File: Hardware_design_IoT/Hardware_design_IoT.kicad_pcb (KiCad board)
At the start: 2 copper layers, 91.2 x 78.8 mm, 90 parts, among them J1 Barrel_Jack_Switch, J2 Prog/Debug, Q1 Q_NPN_BEC_BRT, Q2 Q_NPN_BEC_BRT, Q3 Q_NPN_BEC_BRT, SW1 Input_SW1, SW2 Input_SW2, SW3 PWRKEY_SW, U1 MP1584EN, U2 TLV70033_SOT23-5, U3 STM32L073RZTx, U4 LD39200DPUR, U5 SIM7600E-H, U6 TXB0104RGY, Y1 32.768kHz, Y2 8MHz

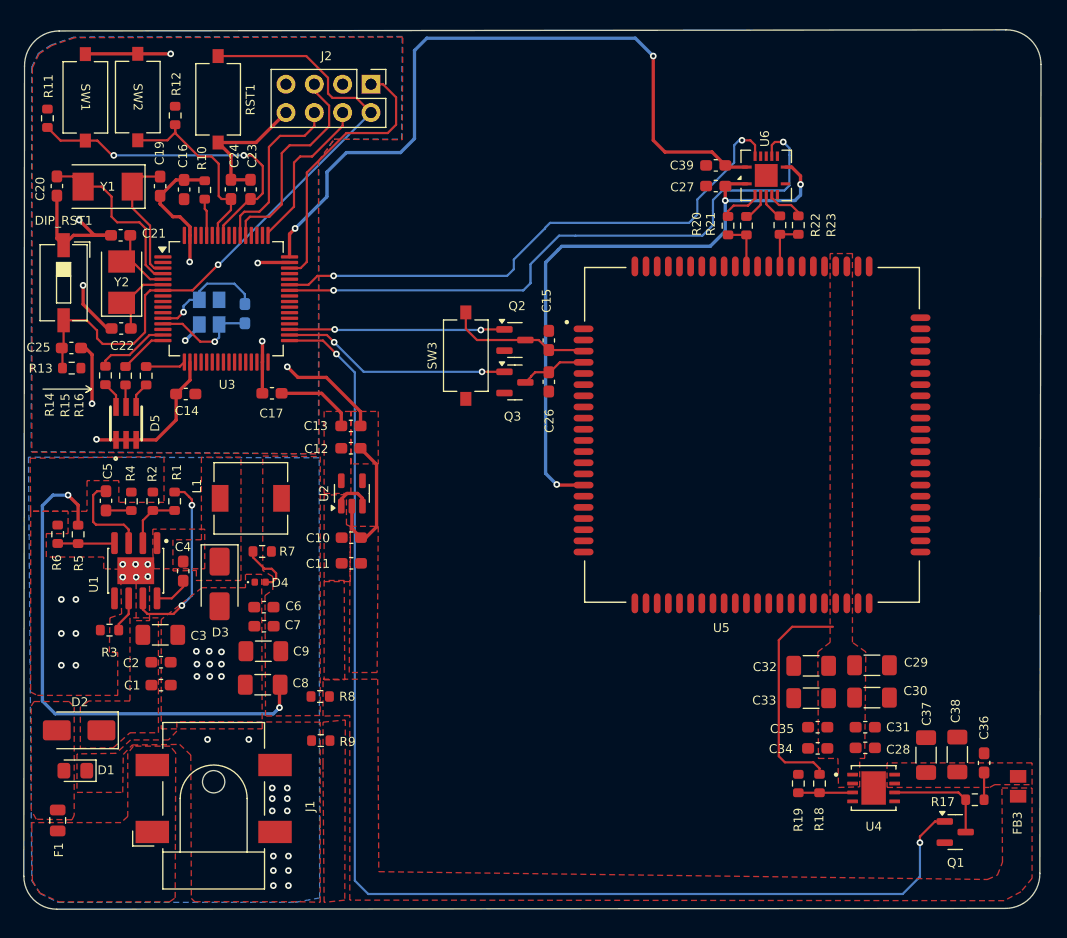
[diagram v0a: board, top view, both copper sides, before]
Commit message: Fin du projet
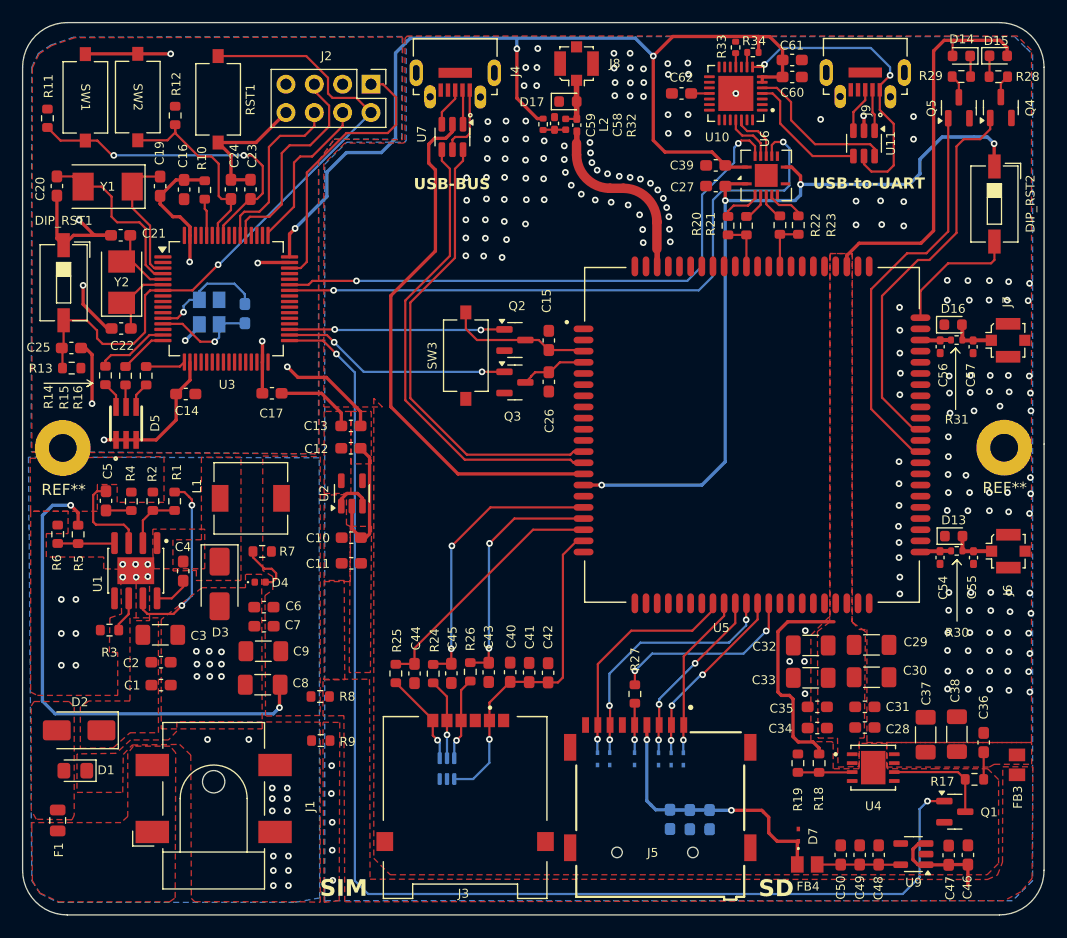
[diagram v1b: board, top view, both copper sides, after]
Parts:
- added C40: 100nF, Capacitor_SMD:C_0603_1608Metric_Pad1.08x0.95mm_HandSolder, F.Cu at (135.4, 116.5)
- added C41: 10nF, Capacitor_SMD:C_0603_1608Metric_Pad1.08x0.95mm_HandSolder, F.Cu at (137.1, 116.5)
- added C42: 10pF, Capacitor_SMD:C_0603_1608Metric_Pad1.08x0.95mm_HandSolder, F.Cu at (138.8, 116.5)
- added C43: 22pF, Capacitor_SMD:C_0603_1608Metric_Pad1.08x0.95mm_HandSolder, F.Cu at (133.5, 116.5)
- added C44: 22pF, Capacitor_SMD:C_0603_1608Metric_Pad1.08x0.95mm_HandSolder, F.Cu at (126.8, 116.6)
- added C45: 22pF, Capacitor_SMD:C_0603_1608Metric_Pad1.08x0.95mm_HandSolder, F.Cu at (130.2, 116.6)
- added C46: 0.1uF, Capacitor_SMD:C_0603_1608Metric_Pad1.08x0.95mm_HandSolder, F.Cu at (176.4, 132.8)
- added C47: 10uF, Capacitor_SMD:C_0603_1608Metric_Pad1.08x0.95mm_HandSolder, F.Cu at (174.7, 132.9)
- added C48: 10uF, Capacitor_SMD:C_0603_1608Metric_Pad1.08x0.95mm_HandSolder, F.Cu at (168.4, 132.8)
- added C49: 0.1uF, Capacitor_SMD:C_0603_1608Metric_Pad1.08x0.95mm_HandSolder, F.Cu at (166.8, 132.8)
- added C50: 22pF, Capacitor_SMD:C_0603_1608Metric_Pad1.08x0.95mm_HandSolder, F.Cu at (165.1, 132.8)
- added C51: 100nF, Capacitor_SMD:C_0603_1608Metric_Pad1.08x0.95mm_HandSolder, B.Cu at (151.5, 129.7)
- added C52: 10uF, Capacitor_SMD:C_0603_1608Metric_Pad1.08x0.95mm_HandSolder, B.Cu at (149.8, 129.7)
- added C53: 10pF, Capacitor_SMD:C_0603_1608Metric_Pad1.08x0.95mm_HandSolder, B.Cu at (153.3, 129.7)
- added C54: DNP, Capacitor_SMD:C_0402_1005Metric_Pad0.74x0.62mm_HandSolder, F.Cu at (173.9, 106.2)
- added C55: DNP, Capacitor_SMD:C_0402_1005Metric_Pad0.74x0.62mm_HandSolder, F.Cu at (176.9, 106.2)
- added C56: DNP, Capacitor_SMD:C_0402_1005Metric_Pad0.74x0.62mm_HandSolder, F.Cu at (174.0, 87.3)
- added C57: DNP, Capacitor_SMD:C_0402_1005Metric_Pad0.74x0.62mm_HandSolder, F.Cu at (176.9, 87.3)
- added C58: 33nF, Capacitor_SMD:C_0402_1005Metric_Pad0.74x0.62mm_HandSolder, F.Cu at (139.4, 67.3)
- added C59: 22pF, Capacitor_SMD:C_0402_1005Metric_Pad0.74x0.62mm_HandSolder, F.Cu at (141.4, 67.4)
- added C60: 4.7uF, Capacitor_SMD:C_0603_1608Metric_Pad1.08x0.95mm_HandSolder, F.Cu at (160.7, 63.1)
- added C61: 100nF, Capacitor_SMD:C_0603_1608Metric_Pad1.08x0.95mm_HandSolder, F.Cu at (160.7, 61.6)
- added C62: 4.7uF, Capacitor_SMD:C_0603_1608Metric_Pad1.08x0.95mm_HandSolder, F.Cu at (150.8, 64.6)
- added D10: ESD9M5.0ST5G, ESD9M5.0ST5G:SODFL1060X40N, B.Cu at (143.2, 124.2)
- added D11: ESD9M5.0ST5G, ESD9M5.0ST5G:SODFL1060X40N, B.Cu at (150.9, 124.2)
- added D12: ESD9M5.0ST5G, ESD9M5.0ST5G:SODFL1060X40N, B.Cu at (149.8, 124.2)
- added D13: TVS, Diode_SMD:D_0603_1608Metric, F.Cu at (175.2, 104.3)
- added D14: Green, LED_SMD:LED_0603_1608Metric, F.Cu at (175.9, 61.2)
- added D15: Red, LED_SMD:LED_0603_1608Metric, F.Cu at (179.2, 61.2)
- added D16: TVS, Diode_SMD:D_0603_1608Metric, F.Cu at (175.1, 85.3)
- added D17: TVS, Diode_SMD:D_0603_1608Metric, F.Cu at (140.6, 65.3)
- added D6: ESD9M5.0ST5G, ESD9M5.0ST5G:SODFL1060X40N, B.Cu at (146.6, 124.2)
- added D7: ESD9M5.0ST5G, ESD9M5.0ST5G:SODFL1060X40N, F.Cu at (161.2, 131.1)
- added D8: ESD9M5.0ST5G, ESD9M5.0ST5G:SODFL1060X40N, B.Cu at (148.7, 124.2)
- added D9: ESD9M5.0ST5G, ESD9M5.0ST5G:SODFL1060X40N, B.Cu at (144.3, 124.2)
- added DIP_RST2: DIP_RST, Button_Switch_SMD:SW_DIP_SPSTx01_Slide_6.7x4.1mm_W6.73mm_P2.54mm_LowProfile_JPin, F.Cu at (178.8, 74.5)
- added FB4: FerriteBead, Ferrite_Bead:BEADC2012X105N, F.Cu at (162.1, 133.7)
- added J3: SMC-216, SMC-216:XUNPU_SMC-216, F.Cu at (131.4, 131.7)
- added J4: UJ2-MIBH2-4-SMT, Micro_USB:CUI_UJ2-MIBH2-4-SMT, F.Cu at (131.8, 64.3)
- added J5: MEM2075-00-140-01-A, MEM2075-00-140-01-A:GCT_MEM2075-00-140-01-A, F.Cu at (148.4, 132.6)
- added J6: Conn_Coaxial, Connector_Coaxial:U.FL_Molex_MCRF_73412-0110_Vertical, F.Cu at (180.1, 105.6)
- added J7: Conn_Coaxial, Connector_Coaxial:U.FL_Molex_MCRF_73412-0110_Vertical, F.Cu at (180.1, 86.7)
- added J8: Conn_Coaxial, Connector_Coaxial:U.FL_Molex_MCRF_73412-0110_Vertical, F.Cu at (141.4, 61.9)
- added J9: UJ2-MIBH2-4-SMT, Micro_USB:CUI_UJ2-MIBH2-4-SMT, F.Cu at (168.6, 64.3)
- added L2: 47nH, Inductor_SMD:L_0402_1005Metric, F.Cu at (140.4, 67.4)
- added Q4: Q_NPN_BEC_BRT, Package_TO_SOT_SMD:SOT-23, F.Cu at (179.4, 65.9)
- added Q5: Q_NPN_BEC_BRT, Package_TO_SOT_SMD:SOT-23, F.Cu at (175.6, 65.9)
- added R24: 22R, Resistor_SMD:R_0603_1608Metric, F.Cu at (128.5, 116.6)
- added R25: 22R, Resistor_SMD:R_0603_1608Metric, F.Cu at (125.2, 116.6)
- added R26: 22R, Resistor_SMD:R_0603_1608Metric, F.Cu at (131.8, 116.4)
- added R27: 22R, Resistor_SMD:R_0603_1608Metric, F.Cu at (146.6, 118.4)
- added R28: 2K, Resistor_SMD:R_0603_1608Metric, F.Cu at (179.2, 63.1)
- added R29: 2K, Resistor_SMD:R_0603_1608Metric, F.Cu at (175.9, 63.1)
- added R30: 22R, Resistor_SMD:R_0402_1005Metric, F.Cu at (175.4, 105.6)
- added R31: 22R, Resistor_SMD:R_0402_1005Metric, F.Cu at (175.4, 86.7)
- added R32: 10R, Resistor_SMD:R_0402_1005Metric, F.Cu at (138.4, 67.4)
- added R33: 10K, Resistor_SMD:R_0402_1005Metric, F.Cu at (155.6, 60.5)
- added R34: 4.7K, Resistor_SMD:R_0402_1005Metric, F.Cu at (157.2, 60.9)
- added REF**: MountingHole_2.5mm_Pad, MountingHole:MountingHole_2.5mm_Pad, F.Cu at (179.7, 96.3)
- added REF**: MountingHole_2.5mm_Pad, MountingHole:MountingHole_2.5mm_Pad, F.Cu at (95.3, 96.4)
- added U10: CP2102-GM, CP2102-GM:QFN50P500X500X100-29N, F.Cu at (155.7, 64.6)
- added U11: USBLC6-2SC6, Package_TO_SOT_SMD:SOT-23-6, F.Cu at (167.1, 69.1)
- added U7: USBLC6-2SC6, Package_TO_SOT_SMD:SOT-23-6, F.Cu at (130.2, 68.5)
- added U8: SMF05CT1G, SMF05CT1G:SOT65P210X110-6N, B.Cu at (129.8, 125.1)
- added U9: LP5907MFX-3.0, Package_TO_SOT_SMD:SOT-23-5, F.Cu at (171.6, 132.8)
- U1: footprint IoT_Library:SOIC127P600X170-9N -> MP1584EN:SOIC127P600X170-9N
- moved FB3 1.93 mm to (180.8, 124.8)
- moved Q1 1.83 mm to (175.3, 129.0)
- moved C34 1.83 mm to (162.9, 121.5)
- moved C35 1.83 mm to (162.9, 119.6)
- moved C28 1.83 mm to (167.2, 121.4)
- moved C30 1.83 mm to (167.8, 116.9)
- moved C31 1.83 mm to (167.2, 119.6)
- moved C32 1.83 mm to (162.4, 114.1)
- moved C33 1.83 mm to (162.4, 117.0)
- moved C37 1.83 mm to (172.7, 122.1)
- moved R17 1.83 mm to (177.0, 126.1)
- moved R18 1.83 mm to (163.1, 124.6)
- moved R19 1.83 mm to (161.2, 124.6)
- moved C29 1.83 mm to (167.8, 114.0)
- moved C36 1.83 mm to (177.9, 122.8)
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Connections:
- U5 pad 12: unconnected-(U5-USB_DN-Pad12) -> /USB_N
- U5 pad 13: unconnected-(U5-USB_DP-Pad13) -> /USB_P
- U5 pad 17: unconnected-(U5-USIM_DATA-Pad17) -> /SIM_DATA
- U5 pad 18: unconnected-(U5-USIM_RST-Pad18) -> /SIM_RST
- U5 pad 19: unconnected-(U5-USIM_CLK-Pad19) -> /SIM_CLK
- U5 pad 20: unconnected-(U5-USIM_VDD-Pad20) -> /SIM_VDD
- U5 pad 27: unconnected-(U5-SDIO_DATA1-Pad27) -> /SD_DATA1
- U5 pad 28: unconnected-(U5-SDIO_DATA2-Pad28) -> /SD_DATA2
- U5 pad 29: unconnected-(U5-SDIO_CMD-Pad29) -> /SD_CMD
- U5 pad 30: unconnected-(U5-SDIO_DATA0-Pad30) -> /SD_DATA0
- U5 pad 31: unconnected-(U5-SDIO_DATA3-Pad31) -> /SD_DATA3
- U5 pad 32: unconnected-(U5-SDIO_CLK-Pad32) -> /SD_CLK
- U5 pad 49: unconnected-(U5-STATUS-Pad49) -> /STATUS
- U5 pad 51: unconnected-(U5-NETLIGHT-Pad51) -> /NETLIGHT
- U5 pad 59: unconnected-(U5-AUX_ANT-Pad59) -> /AUX_ANTENNA
- U5 pad 79: unconnected-(U5-GNSS_ANT-Pad79) -> /GNSS_ANTENNA
- U5 pad 82: unconnected-(U5-MAIN_ANT-Pad82) -> /MAIN_ANTENNA
- U5 pad 85: unconnected-(U5-BOOT_CFG0-Pad85) -> Net-(U5-BOOT_CFG0)
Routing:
- net GND: track 99.3 -> 147.9 mm, vias 9 -> 192
- net /USB_P: track 0.00 -> 42.7 mm
- net /USB_N: track 0.00 -> 42.0 mm
- net /STATUS: track 0.00 -> 36.5 mm
- net /NETLIGHT: track 0.00 -> 35.8 mm
- net /VCC_LTEMODEM: track 20.4 -> 54.3 mm
- net /SIM_VDD: track 0.00 -> 30.1 mm, vias 0 -> 1
- net /3.3V: track 74.7 -> 102.0 mm, vias 3 -> 4
- net /Interfaces/VBUS: track 0.00 -> 27.3 mm, vias 0 -> 2
- net /SIM_DATA: track 0.00 -> 25.5 mm, vias 0 -> 2
- net /3V: track 0.00 -> 24.8 mm, vias 0 -> 2
- net /SD_DATA0: track 0.00 -> 23.2 mm, vias 0 -> 3
- net /SIM_CLK: track 0.00 -> 22.6 mm
- net /SIM_RST: track 0.00 -> 21.7 mm, vias 0 -> 2
- net /SD_DATA1: track 0.00 -> 20.9 mm, vias 0 -> 1
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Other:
- board size 91.2 x 78.8 mm -> 91.6 x 80 mm
- board text added: "SD"
- board text added: "SIM"
- board text added: "USB-BUS"
- board text added: "USB-to-UART"
